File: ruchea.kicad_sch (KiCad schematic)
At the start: 25 parts, among them J11 Conn_01x04, J12 Conn_01x04, J14 Conn_01x03, J17 Conn_01x04, J18 Conn_01x04, J3 Conn_01x03, J4 Conn_01x02, J5 Conn_01x04, J8 Conn_01x03, J9 Conn_01x03, U4 TCA9548APWR, U7 1043

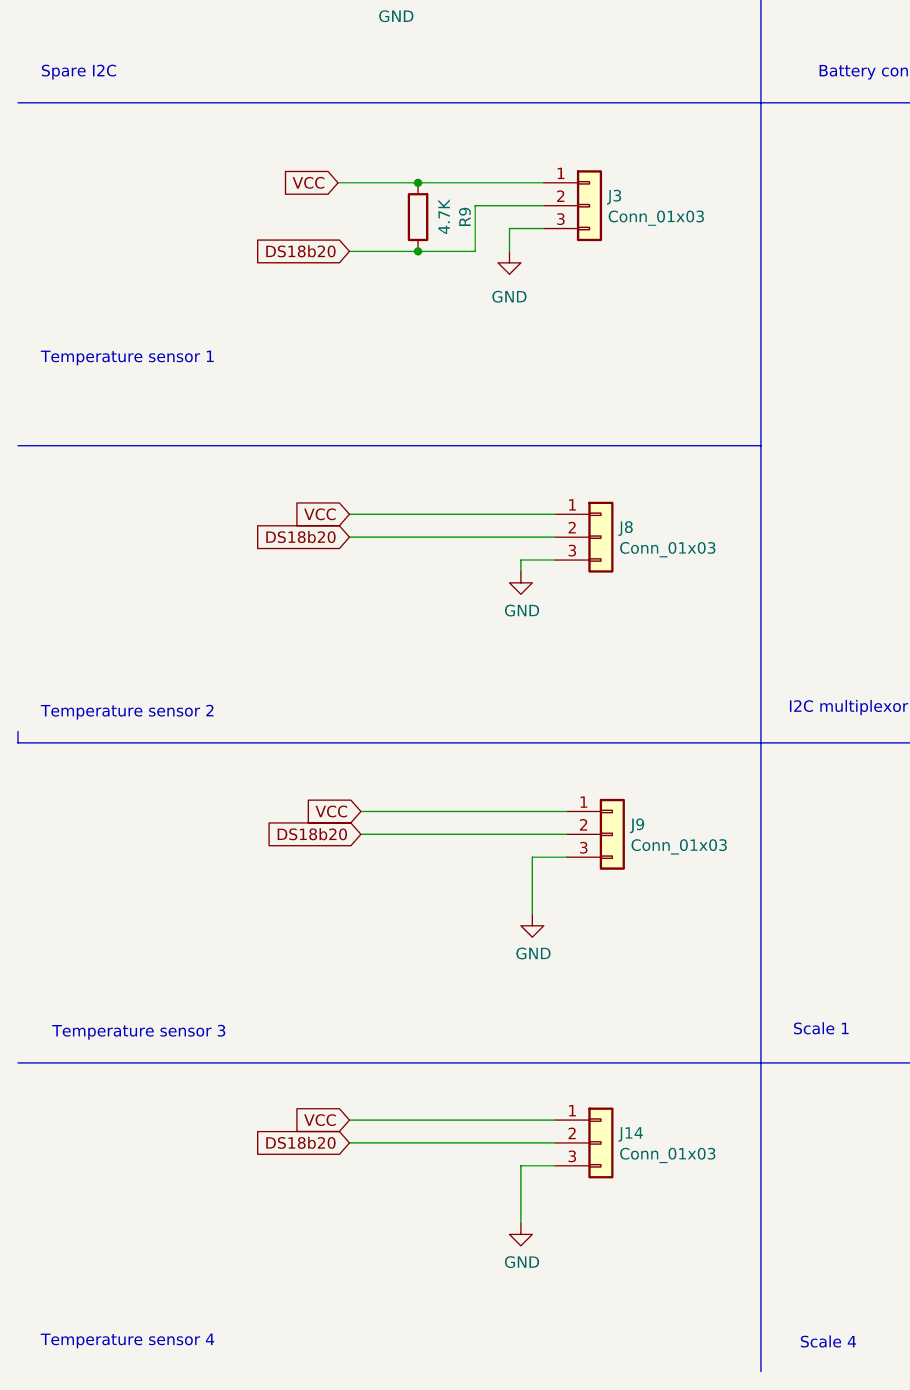
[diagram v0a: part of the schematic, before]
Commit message: update
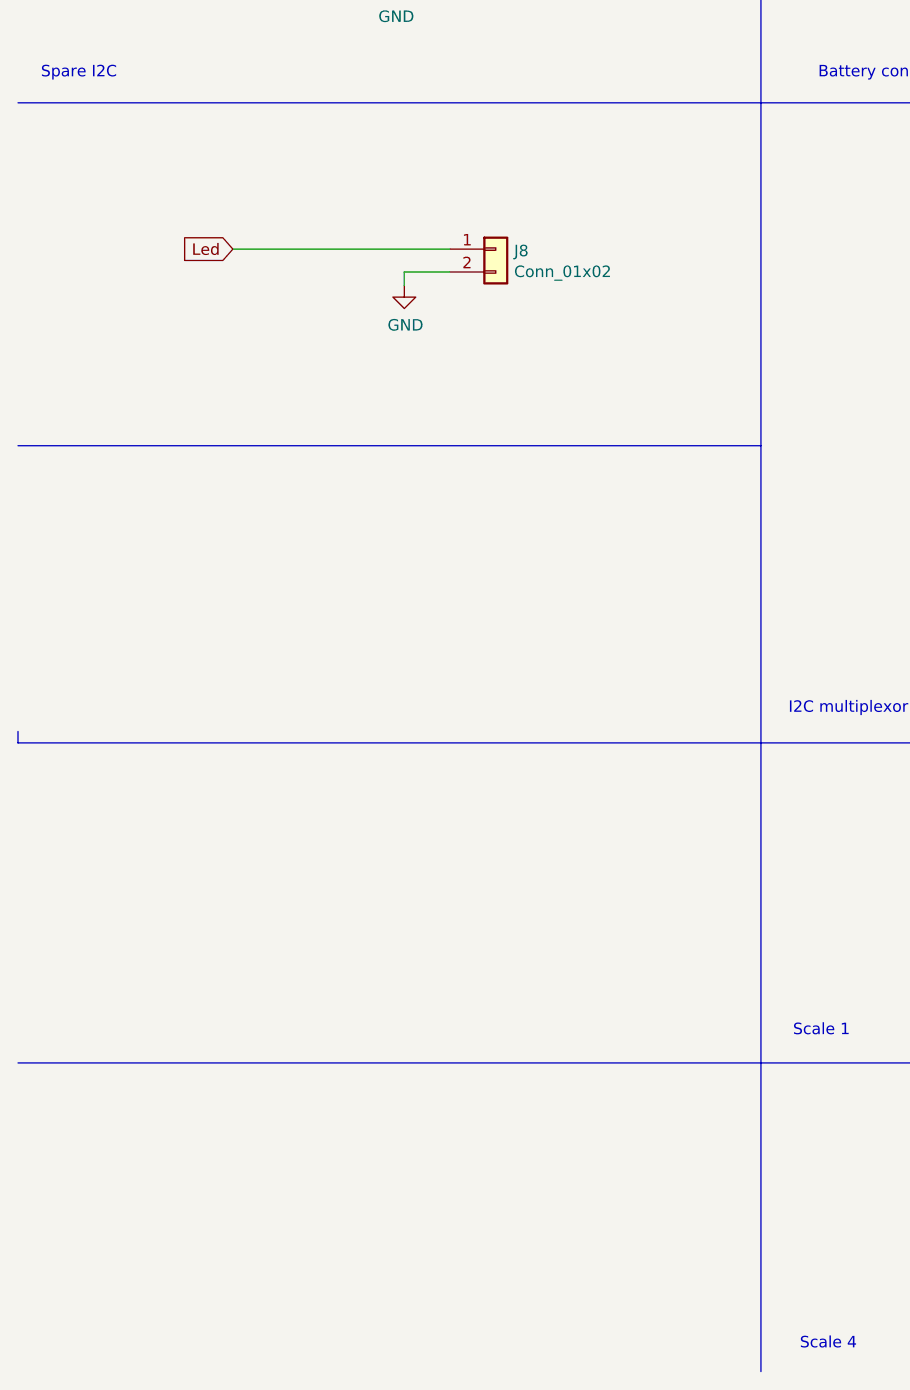
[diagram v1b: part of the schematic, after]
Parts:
- removed J14, J3, J8, J9: Conn_01x03, Connector_JST:JST_PH_B3B-PH-K_1x03_P2.00mm_Vertical, symbol Connector_Generic:Conn_01x03
- removed R9: 4.7K, Resistor_SMD:R_0603_1608Metric, symbol Device:R
- added J8: Conn_01x02, Connector_JST:JST_PH_B2B-PH-K_1x02_P2.00mm_Vertical, symbol Connector_Generic:Conn_01x02
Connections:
- net GND: now also J8.2 (Pin_2)
- new net Led: J8.1 (Pin_1)
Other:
- note removed: "Temperature sensor 1"
- note removed: "Temperature sensor 2"
- note removed: "Temperature sensor 3"
- note removed: "Temperature sensor 4"
